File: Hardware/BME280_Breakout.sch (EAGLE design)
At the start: 11 parts, among them U1 BME280

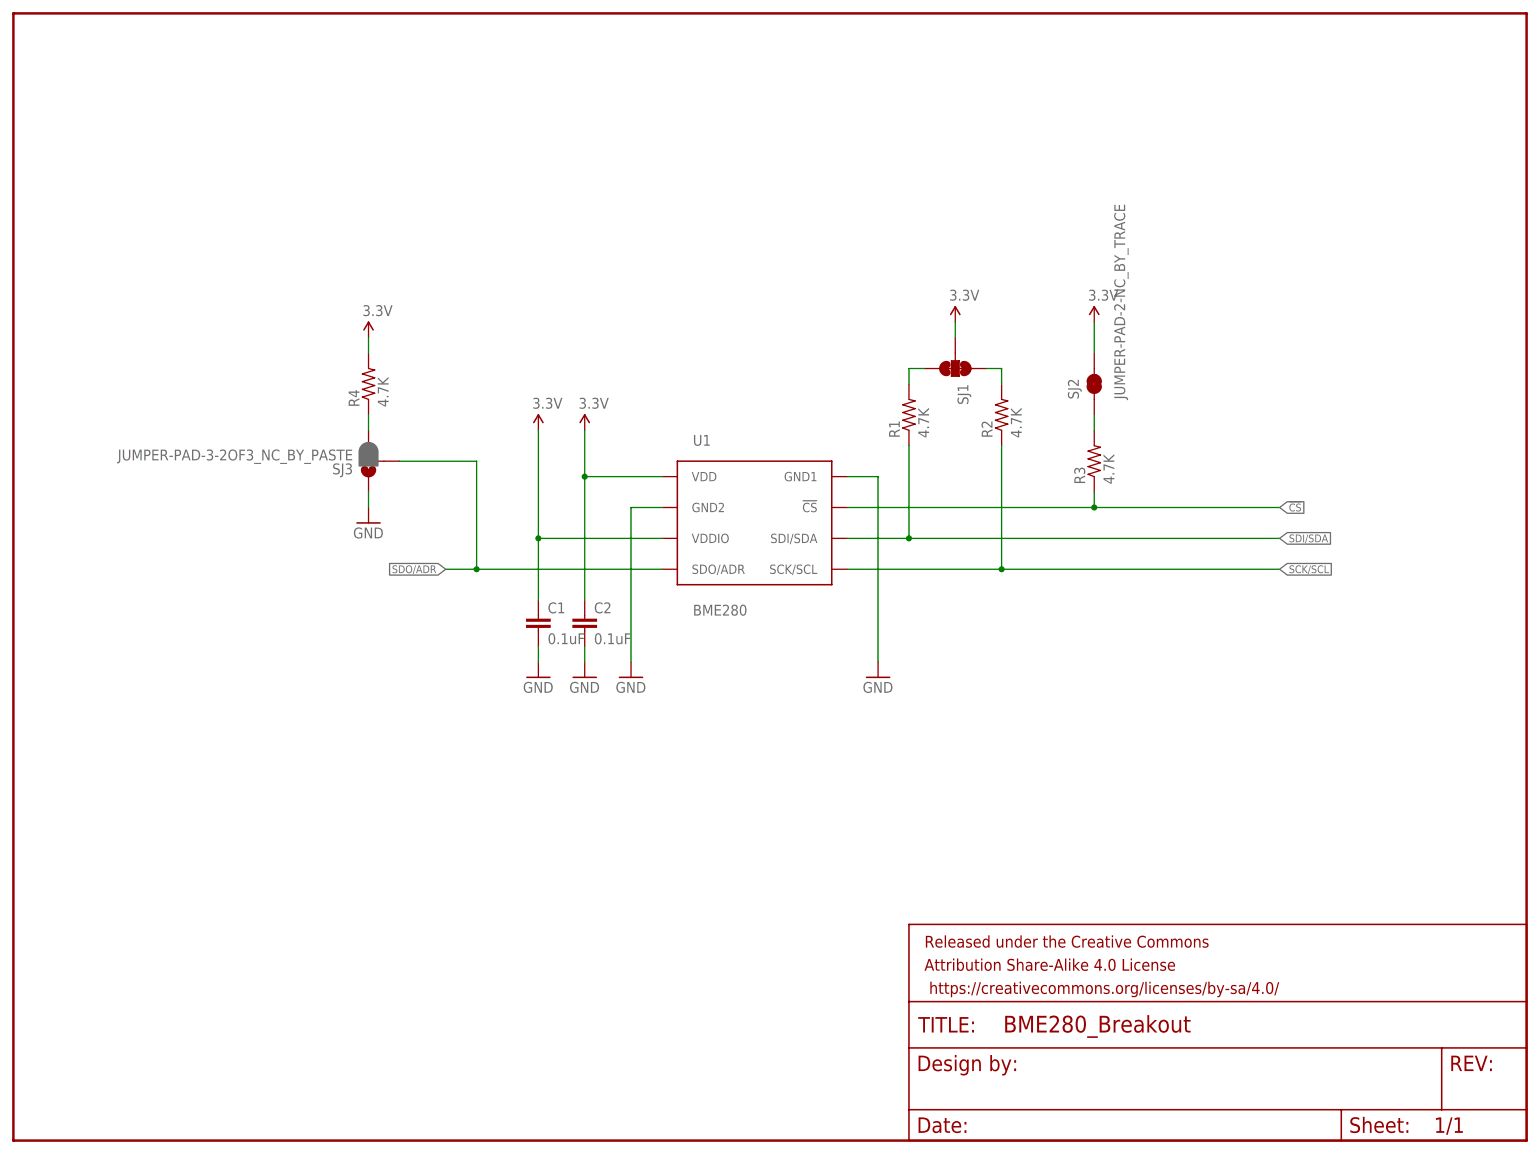
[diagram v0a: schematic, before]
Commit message: Pre-checklist commit
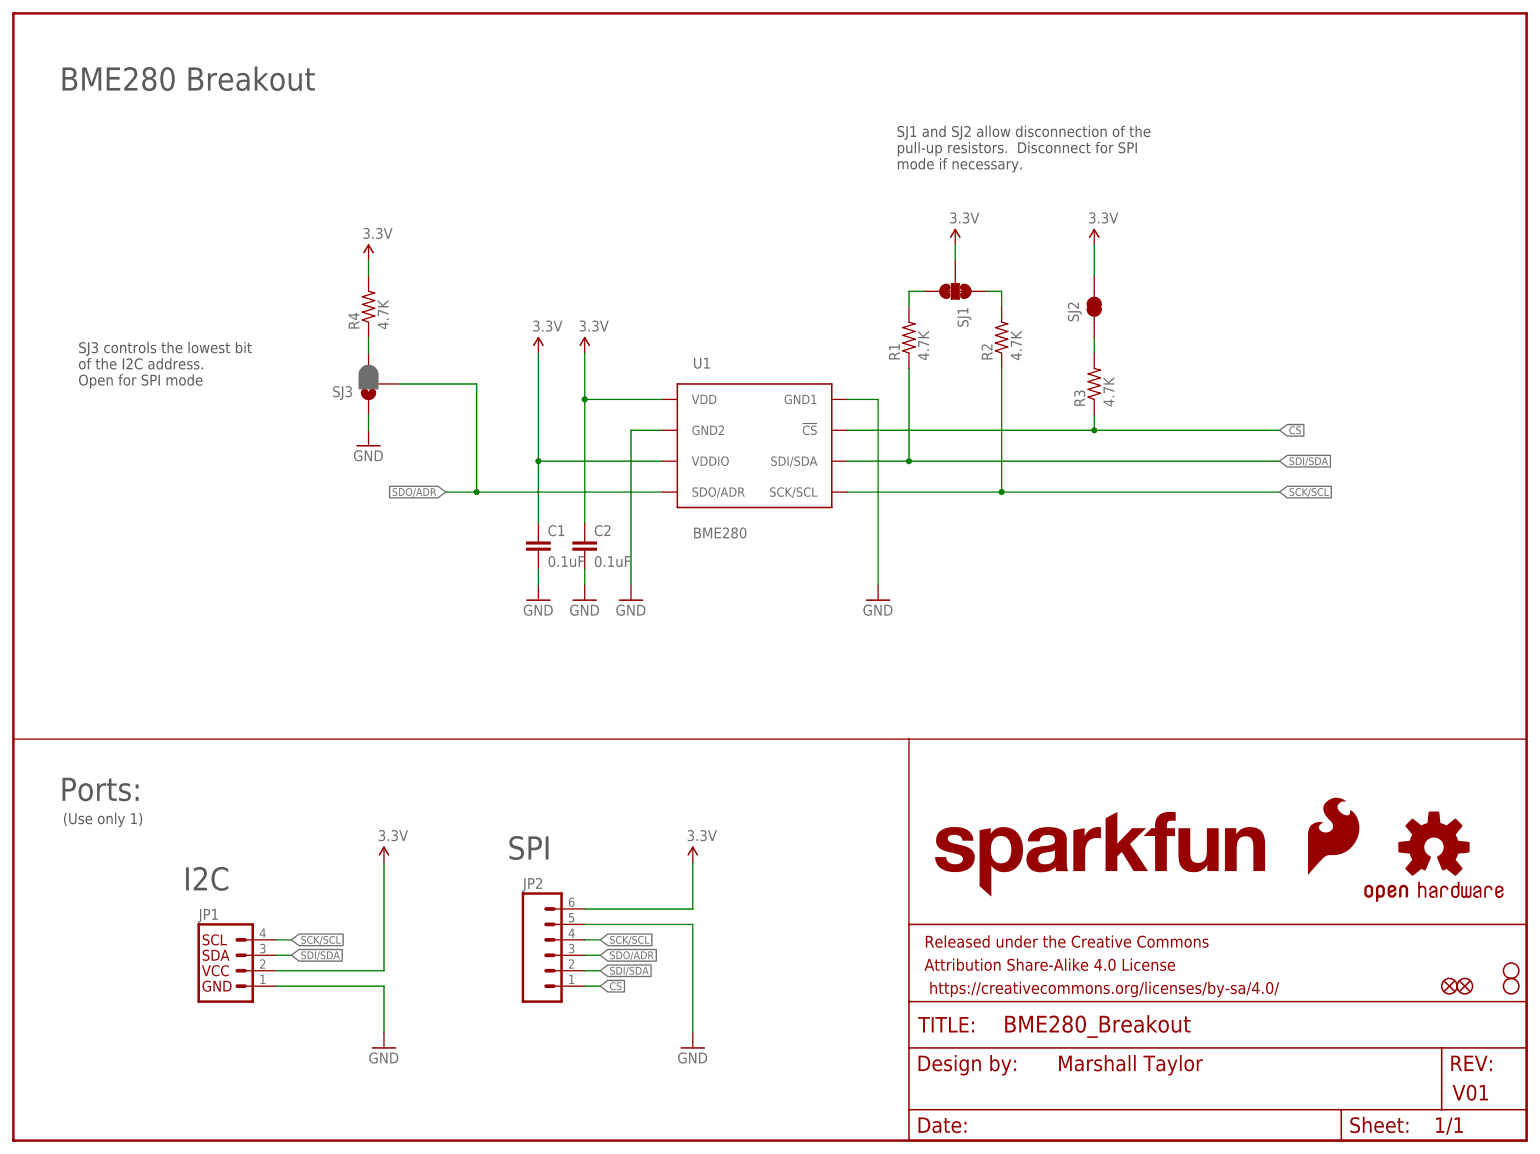
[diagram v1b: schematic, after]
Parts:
- added FID1, FID2: FIDUCIAL1X2, SparkFun-Aesthetics:FIDUCIAL1X2
- added JP1: (no value), SparkFun-Connectors:I2C_STANDARD_NO_SILK
- added JP2: (no value), SparkFun-Connectors:M06NO_SILK_FEMALE_PTH
- added LOGO1: SFE_LOGO_NAME.1_INCH, SparkFun-Aesthetics:SFE_LOGO_NAME.1_INCH
- added LOGO2: SFE_LOGO_FLAME.1_INCH, SparkFun-Aesthetics:SFE_LOGO_FLAME.1_INCH
- added LOGO3: OSHW-LOGOS, SparkFun-Aesthetics:OSHW-LOGOS
- added STANDOFF1, STANDOFF4: STAND-OFF, SparkFun-Electromechanical:STAND-OFF
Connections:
- net !CS: now also JP2.1
- net 3.3V: now also JP1.2, JP2.6
- net GND: now also JP1.1, JP2.5
- net SCK/SCL: now also JP1.4, JP2.4
- net SDI/SDA: now also JP1.3, JP2.2
- net SDO/ADR: now also JP2.3
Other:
- note added: "(Use only 1)"
- note added: "BME280 Breakout"
- note added: "I2C"
- note added: "Marshall Taylor"
- note added: "Ports:"
- note added: "SJ1 and SJ2 allow disconnection of the pull-up resistors. Disconnect for SPI mode if necessary."
- note added: "SJ3 controls the lowest bit of the I2C address. Open for SPI mode"
- note added: "SPI"
- note added: "V01"
- moved on the sheet: C1, C2, R1, R2, R3, R4, SJ1, SJ2, SJ3, U1
